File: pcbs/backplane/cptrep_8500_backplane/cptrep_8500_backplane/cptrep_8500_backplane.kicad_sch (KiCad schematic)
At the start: 5 parts, among them J1 Conn_02x50_Row_Letter_First, J2 Conn_02x50_Row_Letter_First, J3 Conn_02x50_Row_Letter_First, J4 Conn_02x50_Row_Letter_First, J5 Conn_02x50_Row_Letter_First

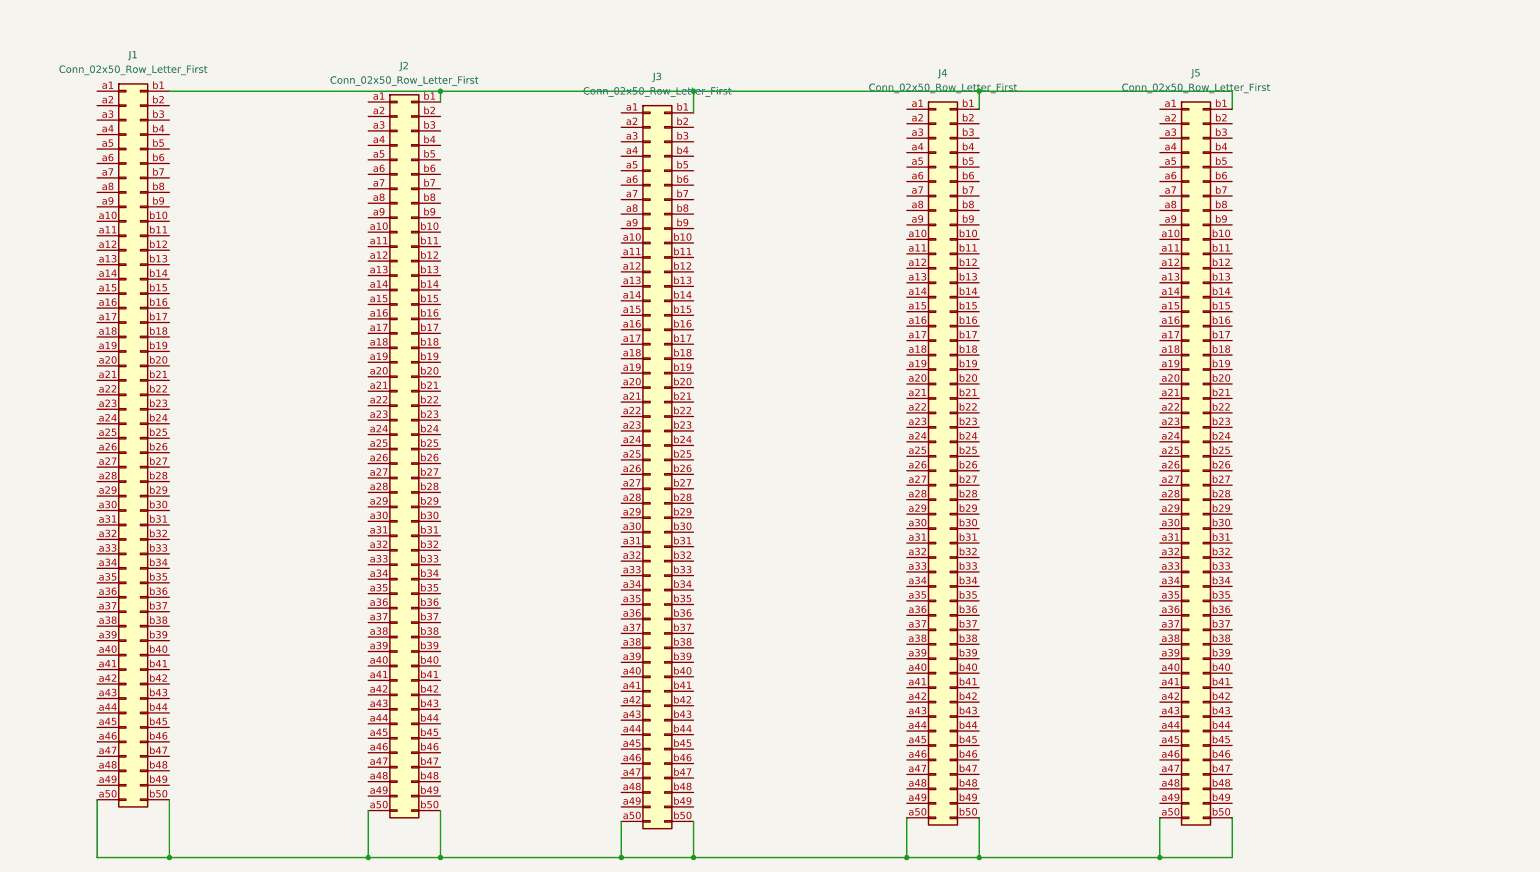
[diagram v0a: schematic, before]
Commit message: "Update"
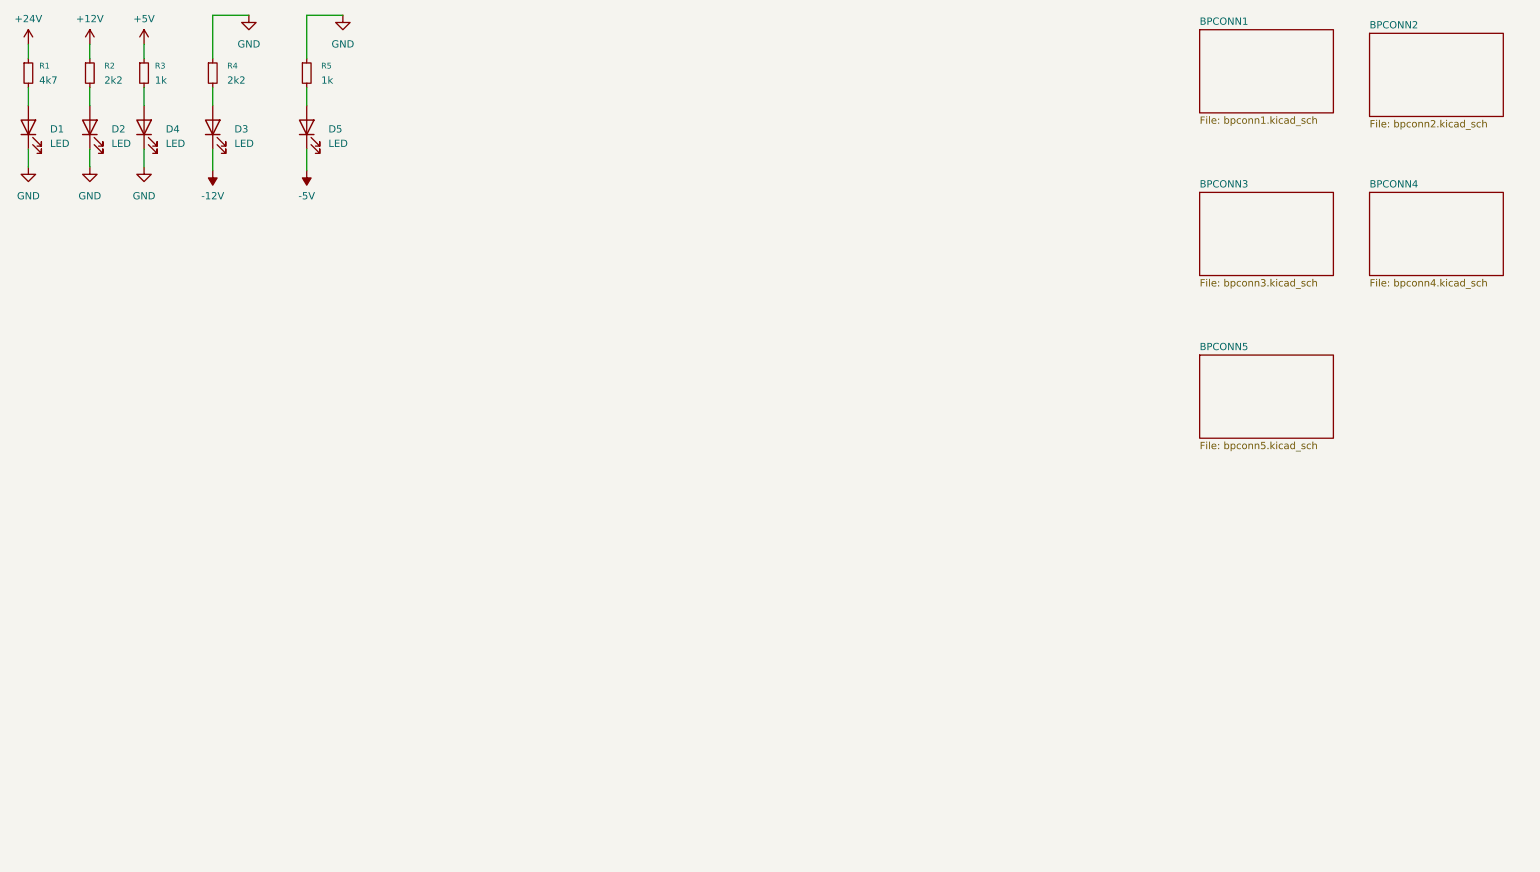
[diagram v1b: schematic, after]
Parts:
- removed J1, J2, J3, J4, J5: Conn_02x50_Row_Letter_First, Connector_Samtec_HLE_THT:Samtec_HLE-150-02-xx-DV-TE_2x50_P2.54mm_Horizontal, symbol Connector_Generic:Conn_02x50_Row_Letter_First
- added D1, D2, D3, D4, D5: LED, symbol Device:LED
- added R1: 4k7, symbol Device:R_Small
- added R2, R4: 2k2, symbol Device:R_Small
- added R3, R5: 1k, symbol Device:R_Small
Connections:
- new net: D3.2 (A), R4.2
- new net: D5.2 (A), R5.2
- new net: D1.2 (A), R1.2
- new net: D2.2 (A), R2.2
- new net: D4.2 (A), R3.2
- new net +12V: R2.1
- new net +24V: R1.1
- new net +5V: R3.1
- new net -12V: D3.1 (K)
- new net -5V: D5.1 (K)
- new net GND: D1.1 (K), D2.1 (K), D4.1 (K), R4.1, R5.1
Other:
- added sheet BPCONN1 (bpconn1.kicad_sch)
- added sheet BPCONN2 (bpconn2.kicad_sch)
- added sheet BPCONN3 (bpconn3.kicad_sch)
- added sheet BPCONN4 (bpconn4.kicad_sch)
- added sheet BPCONN5 (bpconn5.kicad_sch)
